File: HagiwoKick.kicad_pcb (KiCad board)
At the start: 2 copper layers, 30 x 106 mm, 37 parts, among them J1 Tune In, J2 Eurorack_Power_16pin_Shrouded, J3 A. Out, J4 Trig In

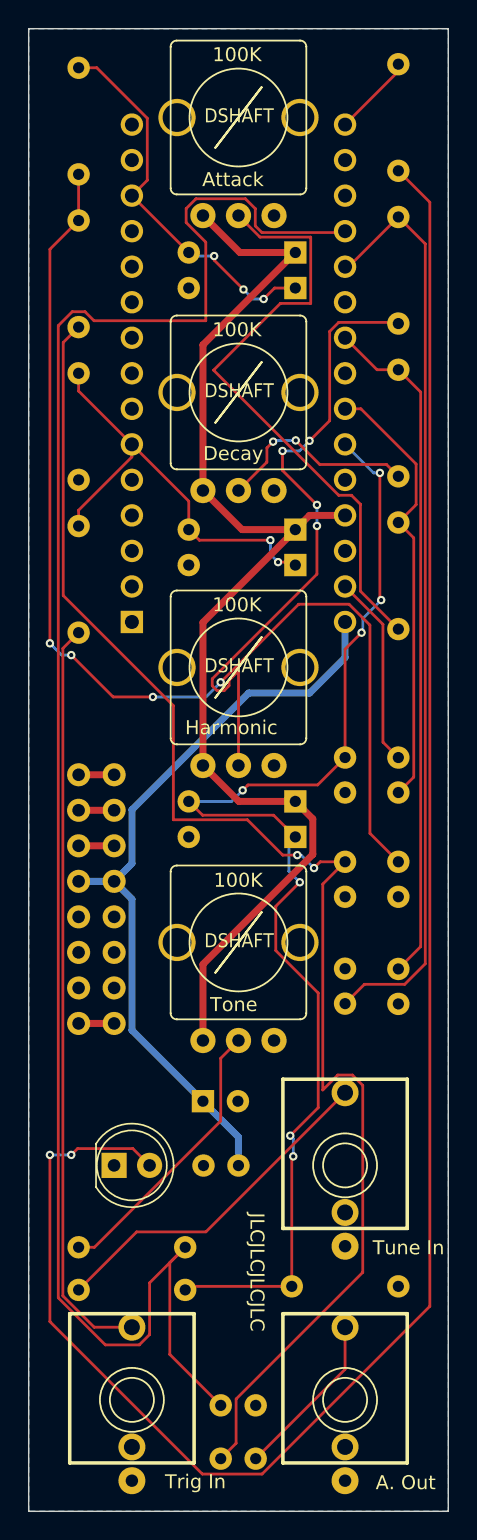
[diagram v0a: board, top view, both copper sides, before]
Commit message: latest updates
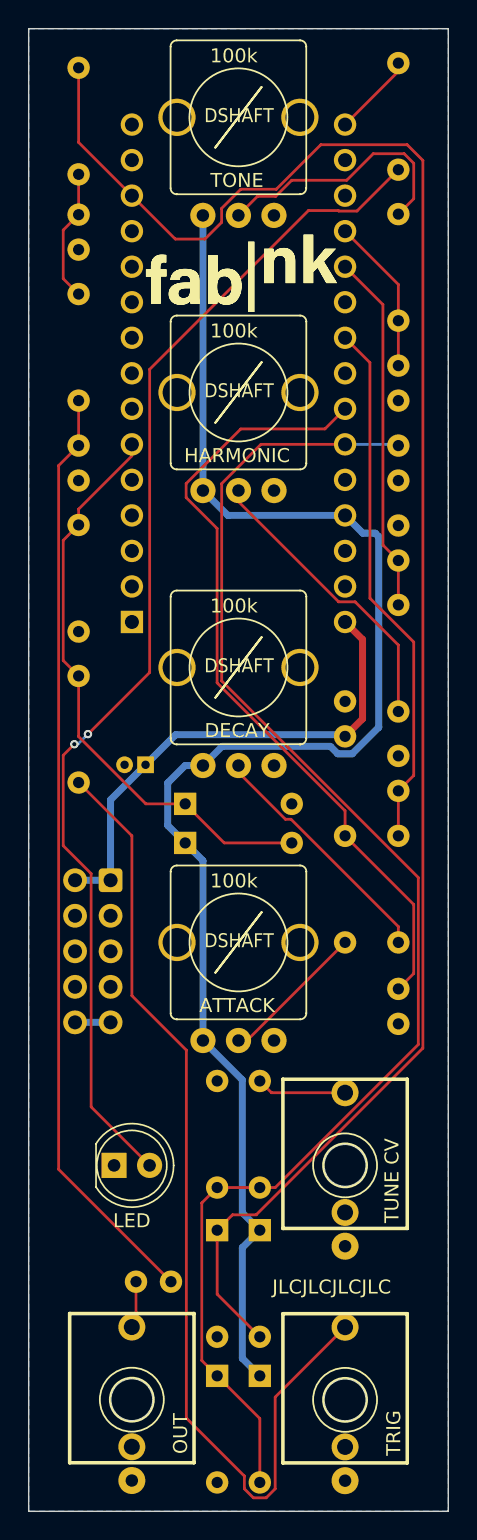
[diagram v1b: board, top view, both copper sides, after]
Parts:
- removed Attack, Decay, Harmonic, Tone: 100K, Library:Pot_9mm_DShaft_RemovedPins4_5
- removed J4: Trig In, Library:EighthInch_PJ398SM_T_TN_S
- added PWR1: Eurorack_Power_10pin_Unshrouded, Library:IDC-Header_2x05_P2.54mm_Vertical_Euro_Power_Striped_ThickerText, B.Cu at (56.9, 111.7)
- added RV1: 100k, Library:Pot_9mm_DShaft_RemovedPins4_5, F.Cu at (66.0, 57.1)
- added RV2: 100k, Library:Pot_9mm_DShaft_RemovedPins4_5, F.Cu at (66.0, 76.8)
- added RV3: 100k, Library:Pot_9mm_DShaft_RemovedPins4_5, F.Cu at (66.0, 116.1)
- added RV4: 100k, Library:Pot_9mm_DShaft_RemovedPins4_5, F.Cu at (66.0, 96.5)
- C1, C2, C3, C4, C5: value 101 -> 100pF
- C10: value 222 -> 2.2nF
- C6: value 104 -> 100nF
- C7: footprint Capacitor_THT:CP_Radial_D5.0mm_P2.50mm -> Capacitor_THT:CP_Radial_D4.0mm_P1.50mm
- C8: value 225 -> 2.2uF
- C9: value 474 -> 470nF
- D1, D2, D3, D4, D5, D6: value B43 -> BAT43; footprint Diode_THT:D_DO-35_SOD27_P7.62mm_Horizontal -> Library:D_DO-35_SOD27_P7.62mm_Horizontal_Widened_No_K
- J1: value Tune In -> TUNE CV; footprint Library:EighthInch_PJ398SM_T_TN_S -> Library:EighthInch_PJ398SM_3mmNPTH
- J2: value Eurorack_Power_16pin_Shrouded -> OUT; footprint PCM_4ms_Connector:Pins_2x08_2.54mm_TH_EuroPower_Shrouded -> Library:EighthInch_PJ398SM_3mmNPTH; moved to F.Cu
- J3: value A. Out -> TRIG; footprint Library:EighthInch_PJ398SM_T_TN_S -> Library:EighthInch_PJ398SM_3mmNPTH
- R1, R10, R2, R3, R4, R5: value 1K -> 1k
- R6, R8: value 100K -> 100k
- R7: value 33K -> 33k
- moved R1 77.3 mm to (77.5, 64.1), turned to -90 degrees
- moved C1 75.4 mm to (77.5, 74.9), turned to -90 degrees
- moved D3 69.9 mm to (67.6, 136.7), turned to -90 degrees
- moved D4 67.6 mm to (64.5, 136.7), turned to -90 degrees
- moved C8 51.6 mm to (54.6, 64.1)
- moved D1 41.1 mm to (67.6, 147.1), turned to -90 degrees
- moved D2 38.9 mm to (64.5, 147.1), turned to -90 degrees
- moved J2 35.9 mm to (58.4, 148.8), turned to -90 degrees
- moved C9 35.3 mm to (54.6, 80.6)
- moved R4 33.3 mm to (77.5, 116.1)
- moved C2 31.9 mm to (77.5, 88.8)
- moved C6 31.6 mm to (73.7, 101.4), turned to 90 degrees
- moved R2 27.7 mm to (77.5, 99.6)
- moved C7 24.4 mm to (59.4, 103.4), turned to 180 degrees
- moved D5 23.7 mm to (62.2, 109.0), turned to 0 degrees
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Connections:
- C10 pad 2: Net-(C10-Pad2) -> Net-(J2-SIG)
- J2 pad 1: Net-(J2-P1) -> Net-(J2-SIG)
- J2 pad 2: Net-(J2-P1) -> unconnected-(J2-SHEILD-Pad2)
- J2 pad 3: Net-(J2-P3) -> GND
- R10 pad 2: Net-(J4-PadT) -> Net-(J3-SIG)
- R5 pad 1: Net-(J1-PadT) -> Net-(J1-SIG)
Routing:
- net A0: track 131.5 -> 11.2 mm
- net D10: track 27.6 -> 129.1 mm, vias 3 -> 0
- net Net-(J3-SIG): track 0.00 -> 71.8 mm
- net Net-(C8-Pad1): track 80.0 -> 9.47 mm, vias 4 -> 0
- net Net-(J4-PadT): track 53.7 -> 0.00 mm
- net Net-(D7-A): track 138.5 -> 85.9 mm
- net A1: track 66.4 -> 25.8 mm
- net Net-(C10-Pad1): track 104.3 -> 66.9 mm, vias 2 -> 0
- net Net-(R3-Pad1): track 44.0 -> 10.5 mm
- net A5: track 31.6 -> 56.9 mm
- net Net-(R2-Pad1): track 46.4 -> 21.2 mm, vias 4 -> 0
- net Net-(J1-PadT): track 24.9 -> 0.00 mm
- net +5V: track 87.3 -> 110.6 mm
- net +12V: track 54.5 -> 36.2 mm
- net GND: track 13.8 -> 0.00 mm
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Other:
- board text added: "SynthLab"
- board text added: "`TR KICK` BY HAGIWO"
- board text added: "github.com/fablabnk/SynthLabProjects"
- board text removed: "`TR KICK` ORIGINAL DESIGN BY HAGIWO"
